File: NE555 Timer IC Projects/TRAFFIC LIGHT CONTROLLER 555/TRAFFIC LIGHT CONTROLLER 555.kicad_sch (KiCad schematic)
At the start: 12 parts, among them U1 LM555xM, U2 4017

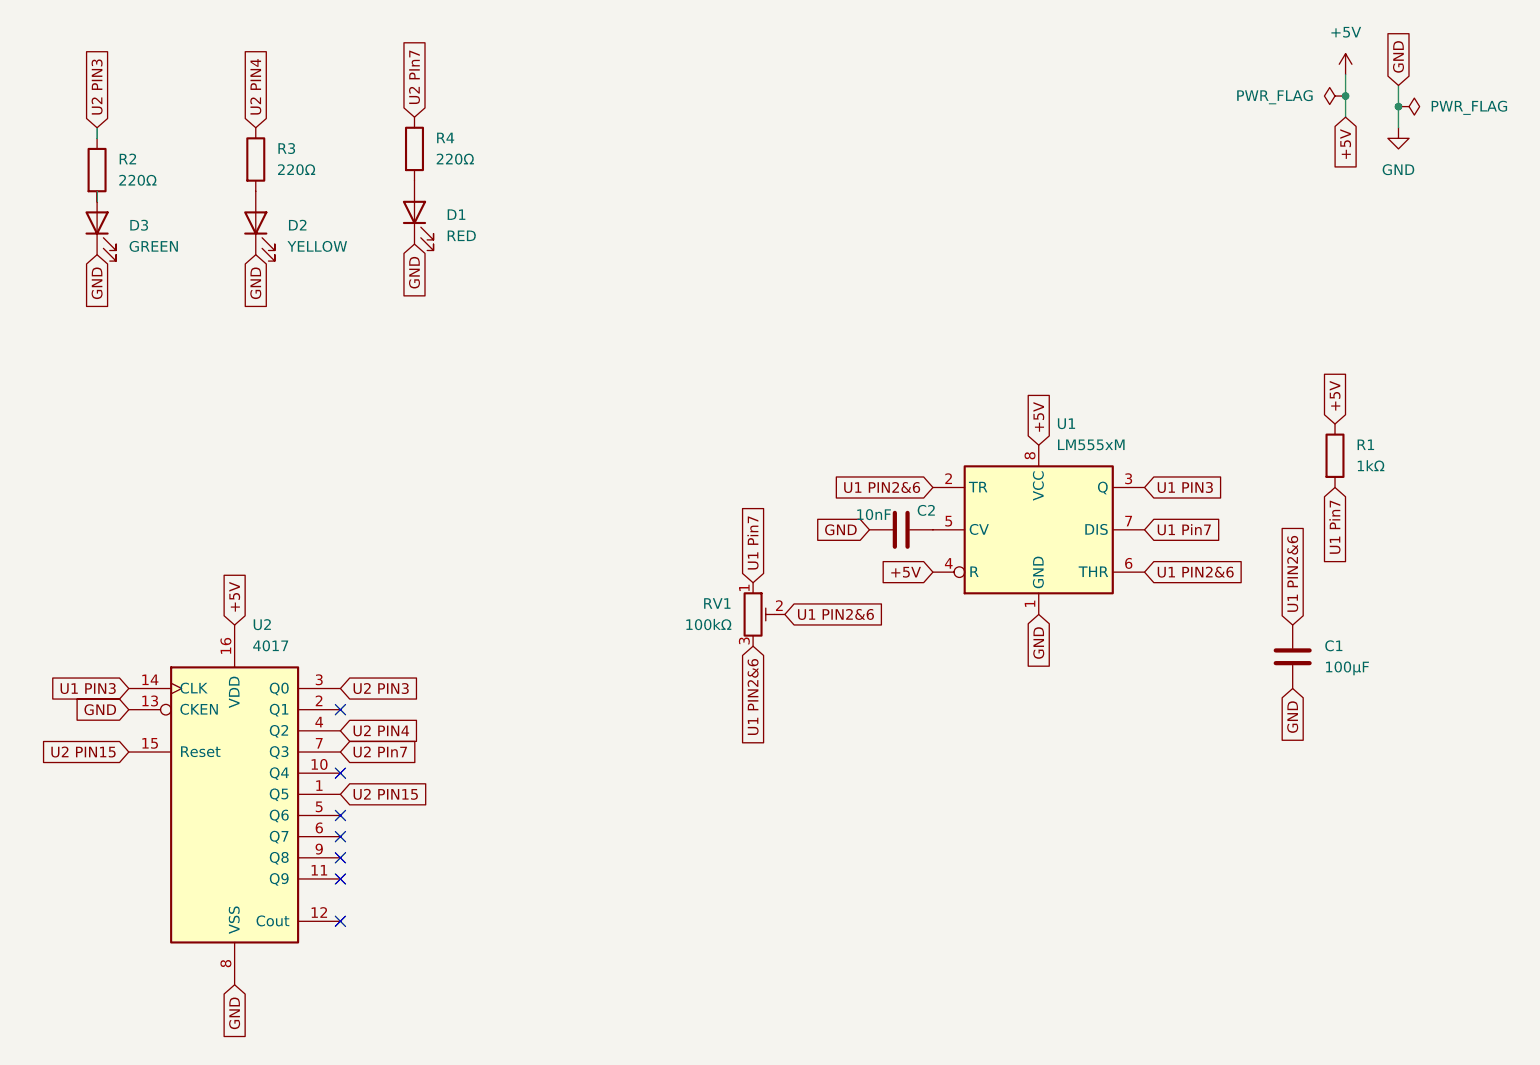
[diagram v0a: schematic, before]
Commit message: Initial Commit
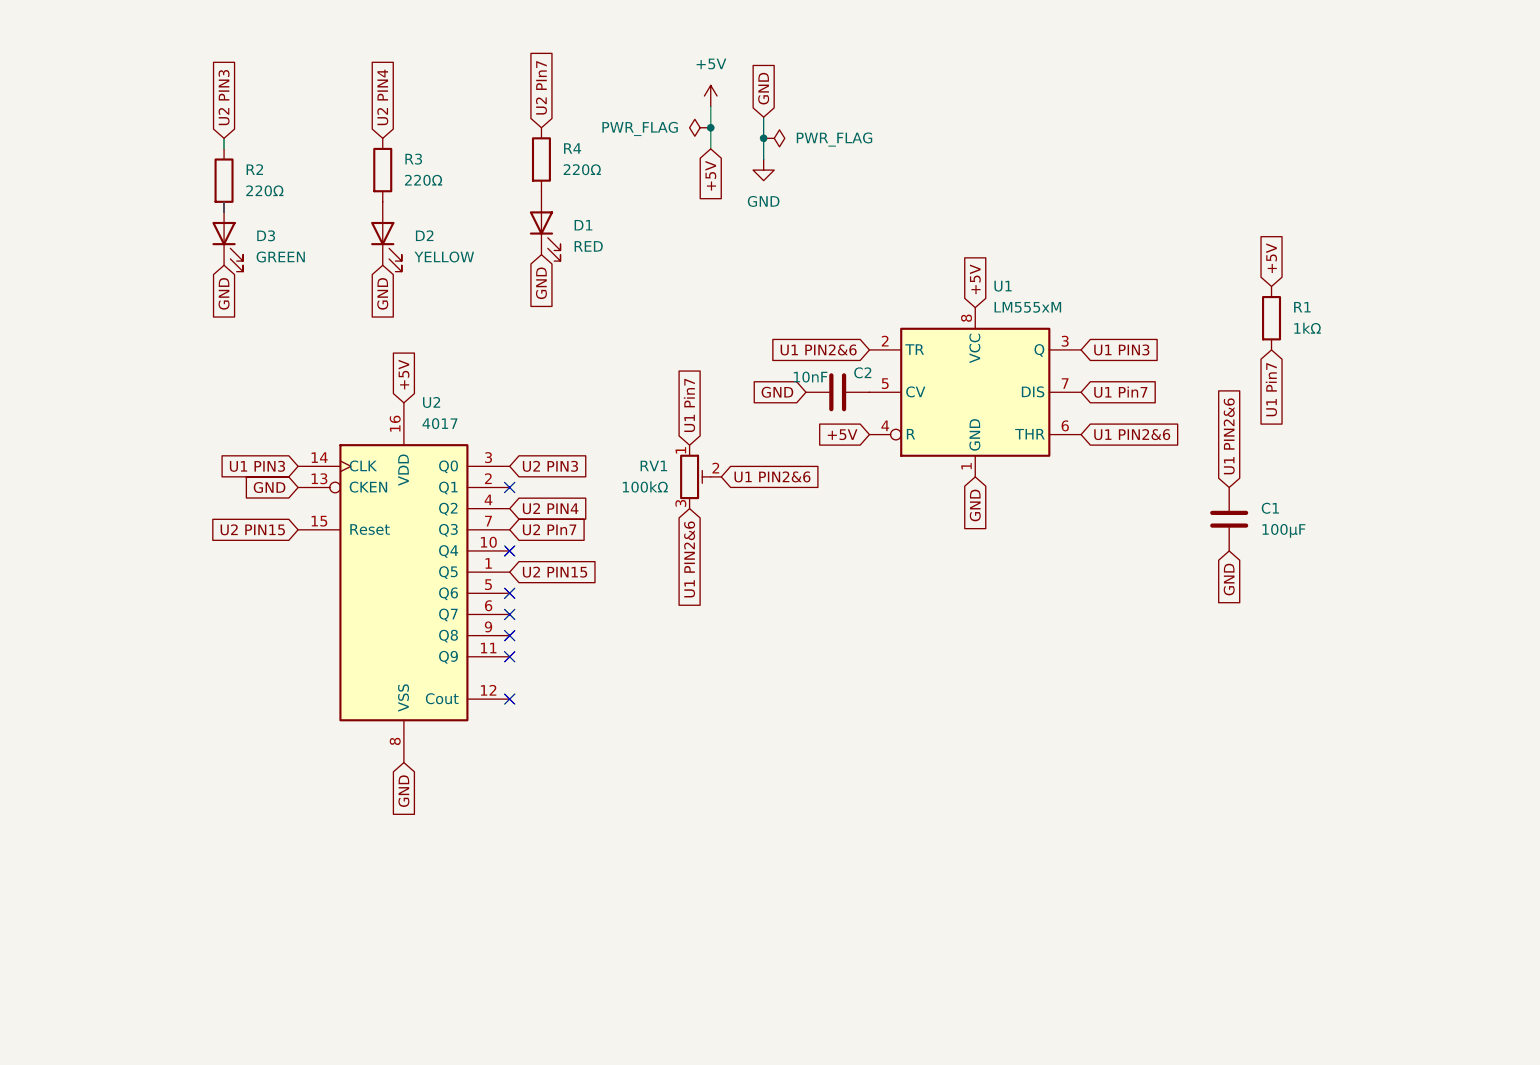
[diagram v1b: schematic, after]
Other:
- moved on the sheet: C1, C2, D1, D2, D3, R1, R2, R3, R4, RV1, U1, U2
